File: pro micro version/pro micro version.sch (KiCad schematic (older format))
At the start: 166 parts, among them SW1 SW_PUSH, U1 ProMicro

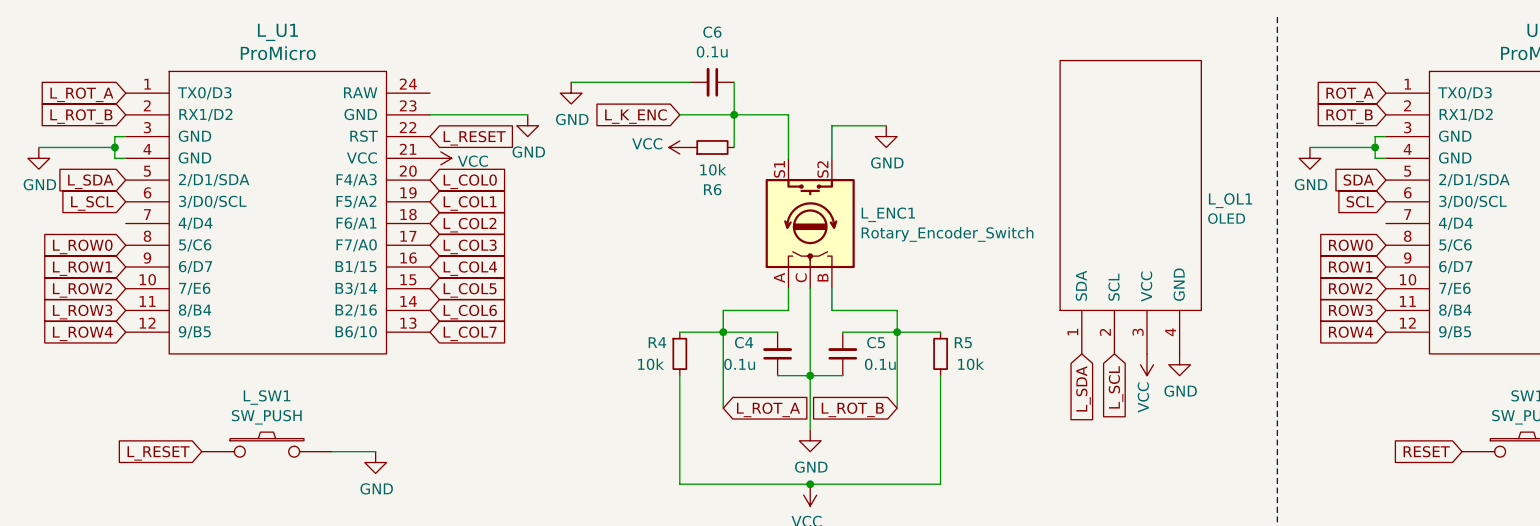
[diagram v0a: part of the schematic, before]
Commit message: finished first routing
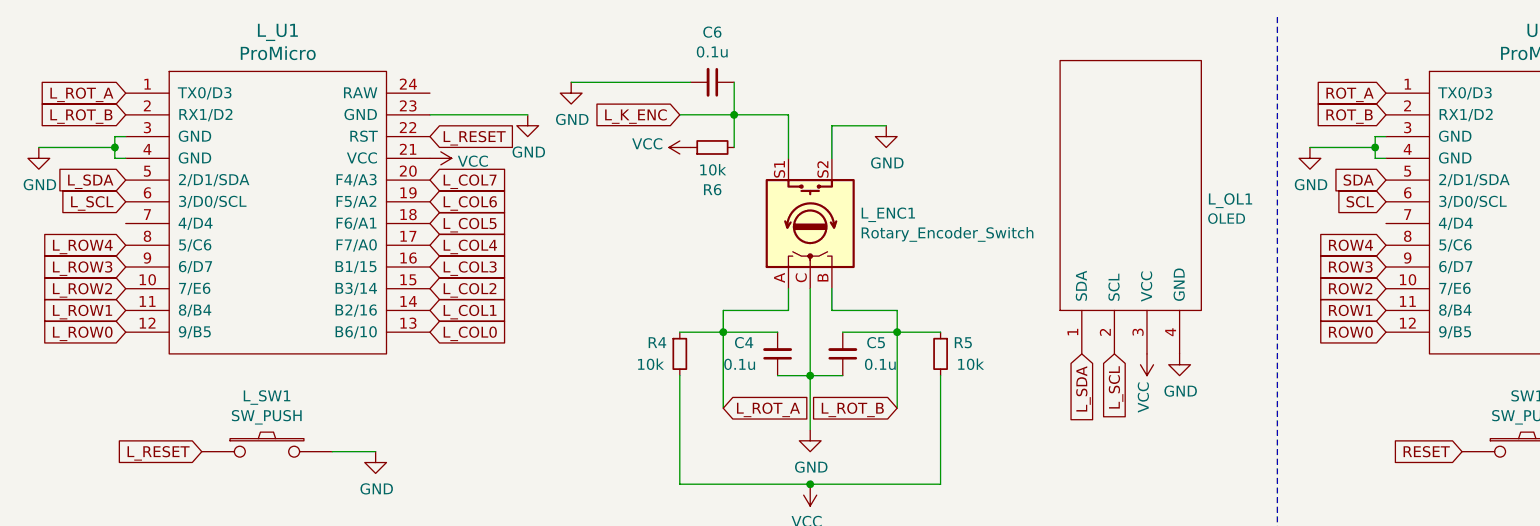
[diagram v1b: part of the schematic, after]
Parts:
- K_Caps1: footprint KeyboardMasterList:MX-1.25U -> KeyboardMasterList:MX-1.75U
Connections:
- net L_COL0: now also L_U1.13 (B6/10); no longer L_U1.20 (F4/A3)
- net L_COL1: now also L_U1.14 (B2/16); no longer L_U1.19 (F5/A2)
- net L_COL2: now also L_U1.15 (B3/14); no longer L_U1.18 (F6/A1)
- net L_COL3: now also L_U1.16 (B1/15); no longer L_U1.17 (F7/A0)
- net L_COL4: now also L_U1.17 (F7/A0); no longer L_U1.16 (B1/15)
- net L_COL5: now also L_U1.18 (F6/A1); no longer L_U1.15 (B3/14)
- net L_COL6: now also L_U1.19 (F5/A2); no longer L_U1.14 (B2/16)
- net L_COL7: now also L_U1.20 (F4/A3); no longer L_U1.13 (B6/10)
- net L_ROW0: now also L_U1.12 (9/B5); no longer L_U1.8 (5/C6)
- net L_ROW1: now also L_U1.11 (8/B4); no longer L_U1.9 (6/D7)
- net L_ROW3: now also L_U1.9 (6/D7); no longer L_U1.11 (8/B4)
- net L_ROW4: now also L_U1.8 (5/C6); no longer L_U1.12 (9/B5)
- net ROW0: now also U1.12 (9/B5); no longer U1.8 (5/C6)
- net ROW1: now also U1.11 (8/B4); no longer U1.9 (6/D7)
- net ROW3: now also U1.9 (6/D7); no longer U1.11 (8/B4)
- net ROW4: now also U1.8 (5/C6); no longer U1.12 (9/B5)
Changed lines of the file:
@@
 Text GLabel 1000 950  0    50   Input ~ 0
 L_ROT_B
-Text GLabel 1000 1550 0    50   Input ~ 0
+Text GLabel 1000 1950 0    50   Input ~ 0
 L_ROW0
-Text GLabel 1000 1650 0    50   Input ~ 0
+Text GLabel 1000 1850 0    50   Input ~ 0
 L_ROW1
 Text GLabel 1000 1750 0    50   Input ~ 0
 L_ROW2
-Text GLabel 1000 1850 0    50   Input ~ 0
+Text GLabel 1000 1650 0    50   Input ~ 0
 L_ROW3
-Text GLabel 1000 1950 0    50   Input ~ 0
+Text GLabel 1000 1550 0    50   Input ~ 0
 L_ROW4
+Text GLabel 2400 1950 2    50   Input ~ 0
+L_COL0
+Text GLabel 2400 1850 2    50   Input ~ 0
+L_COL1
+Text GLabel 2400 1750 2    50   Input ~ 0
+L_COL2
+Text GLabel 2400 1650 2    50   Input ~ 0
+L_COL3
+Text GLabel 2400 1550 2    50   Input ~ 0
+L_COL4
+Text GLabel 2400 1450 2    50   Input ~ 0
+L_COL5
+Text GLabel 2400 1350 2    50   Input ~ 0
+L_COL6
 Text GLabel 2400 1250 2    50   Input ~ 0
-L_COL0
-Text GLabel 2400 1350 2    50   Input ~ 0
-L_COL1
-Text GLabel 2400 1450 2    50   Input ~ 0
-L_COL2
-Text GLabel 2400 1550 2    50   Input ~ 0
-L_COL3
-Text GLabel 2400 1650 2    50   Input ~ 0
-L_COL4
-Text GLabel 2400 1750 2    50   Input ~ 0
-L_COL5
-Text GLabel 2400 1850 2    50   Input ~ 0
-L_COL6
-Text GLabel 2400 1950 2    50   Input ~ 0
 L_COL7
 $Comp
@@
 Text GLabel 6800 950  0    50   Input ~ 0
 ROT_B
-Text GLabel 6800 1550 0    50   Input ~ 0
+Text GLabel 6800 1950 0    50   Input ~ 0
 ROW0
-Text GLabel 6800 1650 0    50   Input ~ 0
+Text GLabel 6800 1850 0    50   Input ~ 0
 ROW1
 Text GLabel 6800 1750 0    50   Input ~ 0
 ROW2
-Text GLabel 6800 1850 0    50   Input ~ 0
+Text GLabel 6800 1650 0    50   Input ~ 0
 ROW3
-Text GLabel 6800 1950 0    50   Input ~ 0
+Text GLabel 6800 1550 0    50   Input ~ 0
 ROW4
 Text GLabel 8200 1250 2    50   Input ~ 0
@@
 F 0 "K_Caps1" H 1733 4973 60  0000 C CNN
 F 1 "MX-NoLED" H 1733 4899 20  0000 C CNN
-F 2 "KeyboardMasterList:MX-1.25U" H 1075 4725 60  0001 C CNN
+F 2 "KeyboardMasterList:MX-1.75U" H 1075 4725 60  0001 C CNN
 F 3 "" H 1075 4725 60  0001 C CNN
 	1    1700 4750
